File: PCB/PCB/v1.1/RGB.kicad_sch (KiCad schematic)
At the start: 36 parts, among them J26 , J27 , J28 , J29 

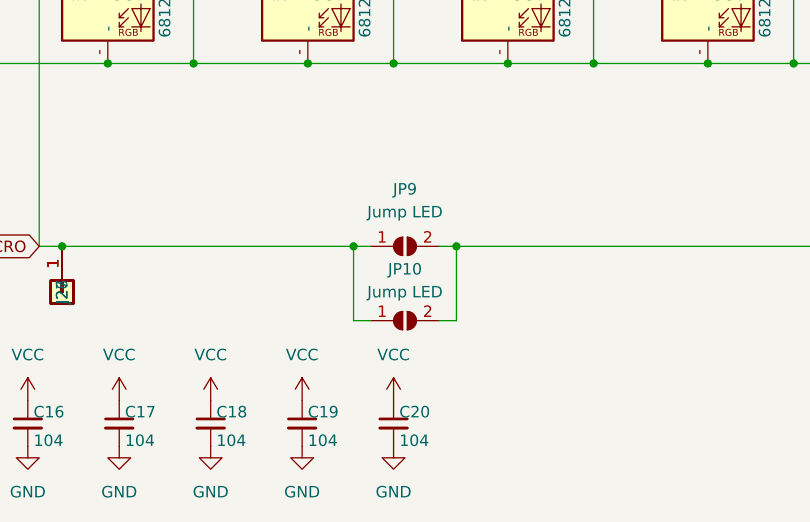
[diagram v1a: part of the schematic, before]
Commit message: Update PCB
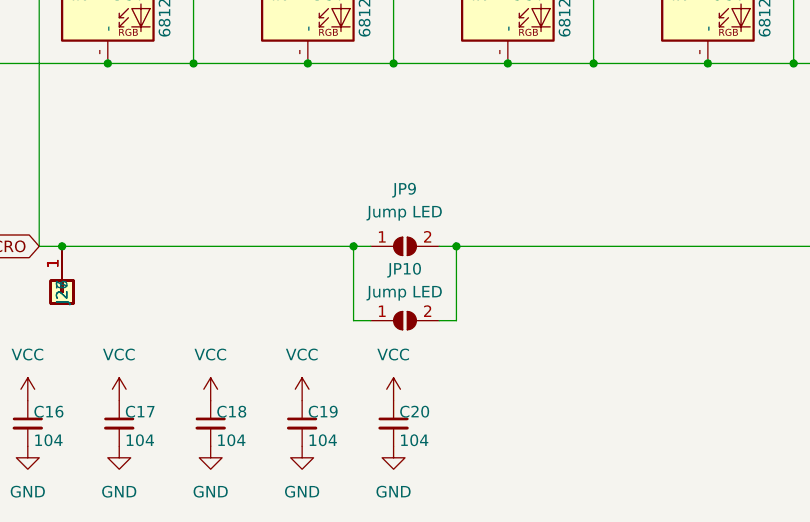
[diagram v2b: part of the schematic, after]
